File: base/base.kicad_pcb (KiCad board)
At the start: 2 copper layers, 73.7 x 78.7 mm, 16 parts, among them J1 POWER_OUTPUT-, J2 POWER_OUTPUT-, J3 POWER_OUTPUT+, J4 POWER_OUTPUT+, J5 POWER_INPUT+, J6 POWER_INPUT-, J7 FAN_3pin, J8 FAN_4pin, SW1 VSELECT, U1 LM7812_TO220

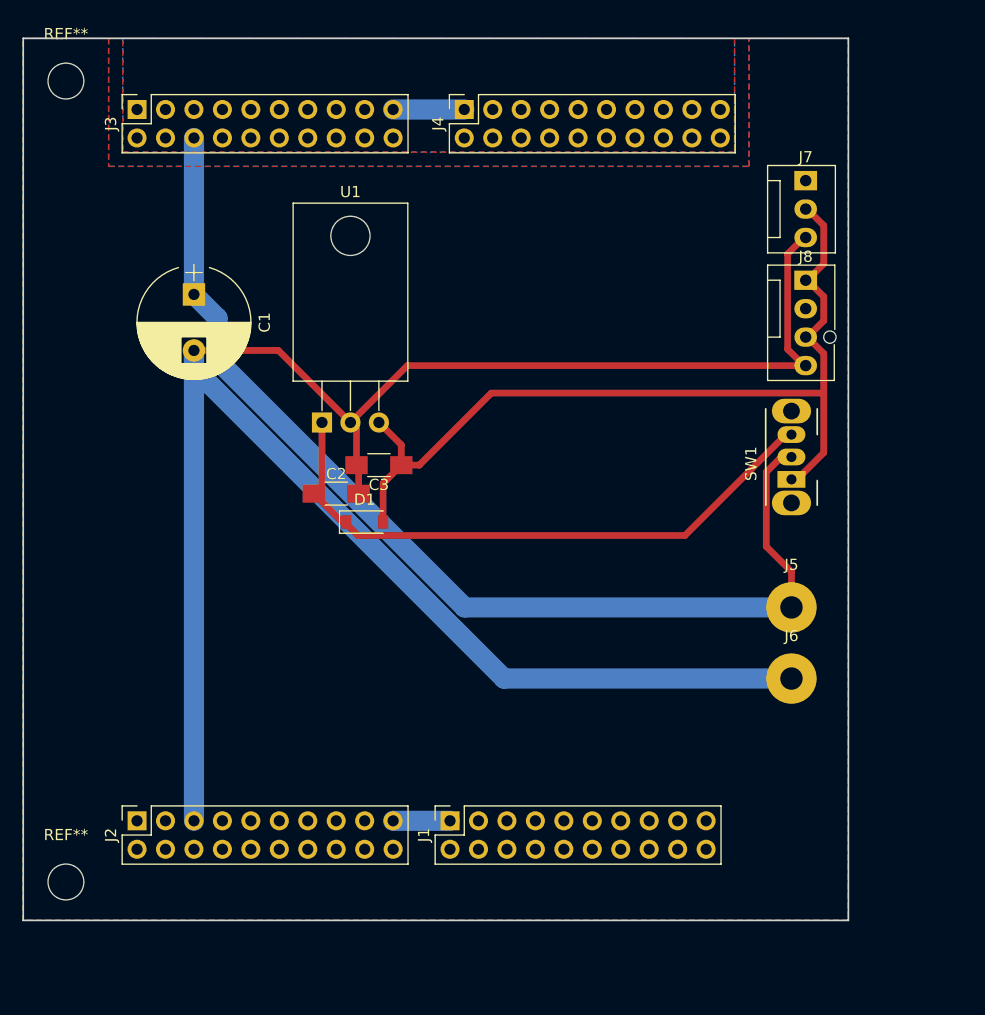
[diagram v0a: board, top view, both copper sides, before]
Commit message: PCBのガーバー出力
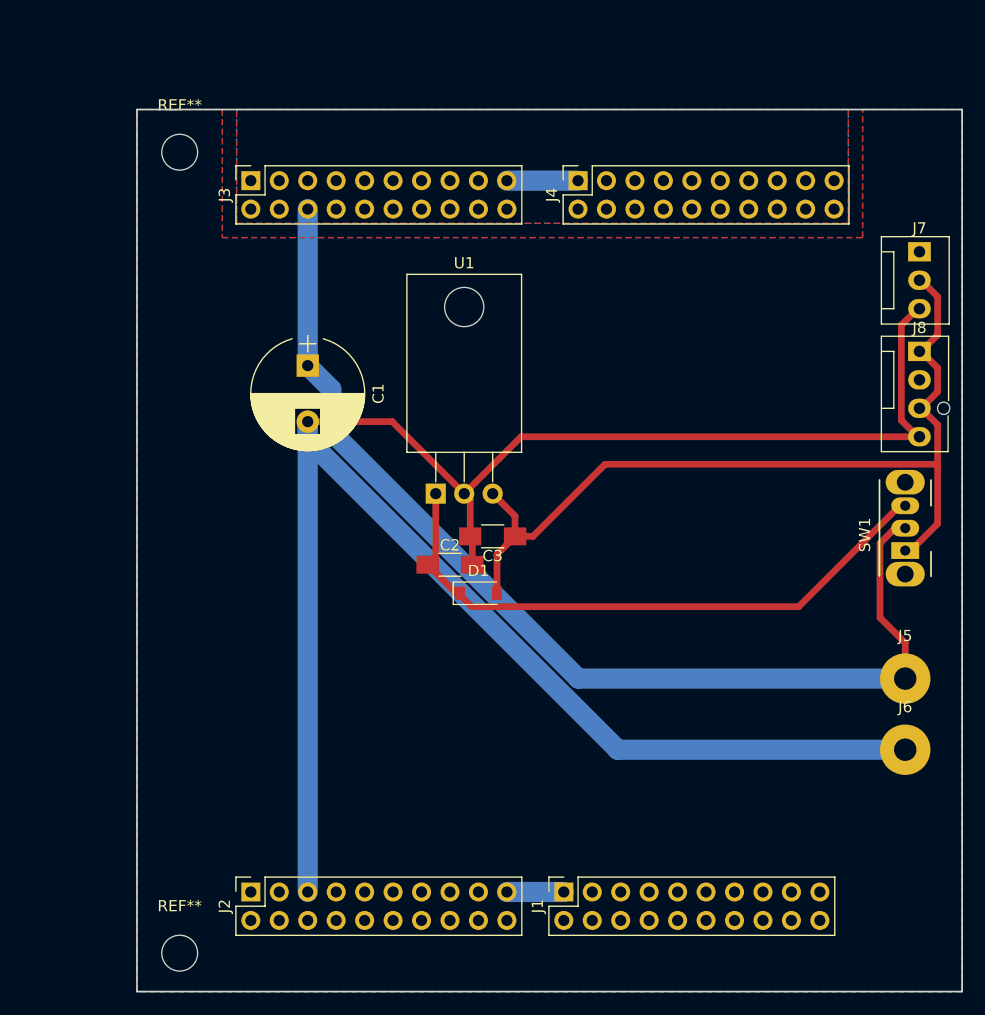
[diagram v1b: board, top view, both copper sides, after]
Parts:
- moved J7 12.0 mm to (69.8, 12.7)
- moved J8 12.0 mm to (69.8, 21.6)
- moved REF** 12.0 mm to (3.81, 75.3)
- moved D1 12.0 mm to (30.5, 43.2)
- moved J4 12.0 mm to (39.4, 6.35)
- moved C1 12.0 mm to (15.2, 22.9)
- moved C2 12.0 mm to (27.9, 40.6)
- moved C3 12.0 mm to (31.7, 38.1)
- moved J2 12.0 mm to (10.2, 69.9)
- moved J3 12.0 mm to (10.2, 6.35)
- moved REF** 12.0 mm to (3.81, 3.81)
- moved J1 12.0 mm to (38.1, 69.9)
- moved J6 12.0 mm to (68.6, 57.2)
- moved U1 12.0 mm to (26.7, 34.3)
- moved J5 12.0 mm to (68.6, 50.8)
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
